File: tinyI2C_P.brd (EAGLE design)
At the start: 80.8 x 80 mm, 224 parts, among them IC1 74ABT125BQ, IC10 74ABT125BQ, IC11 TPS76318, IC12 74ABT125BQ, IC13 TPS76318, IC14 74ABT125BQ, IC15 TPS76318, IC16 74ABT125BQ, IC2 TPS76318, IC3 TPS76318, IC4 74ABT125BQ, IC5 TPS76318, IC6 74ABT125BQ, IC7 TPS76318, IC8 74ABT125BQ, IC9 TPS76318, U1 LPC824M201JHI33, U2 LPC824M201JHI33, U3 LPC824M201JHI33, U4 LPC824M201JHI33, U5 LPC824M201JHI33, U6 LPC824M201JHI33, U7 LPC824M201JHI33, U8 LPC824M201JHI33, X1 TSW-112-02-S-S, X10 TSW-112-02-S-S, X11 TSW-112-02-S-S, X12 TSW-102-02-S-S, X13 TSW-106-02-S-S-RA, X14 TSW-112-02-S-S, X15 TSW-112-02-S-S, X16 TSW-102-02-S-S, X17 TSW-106-02-S-S-RA, X18 TSW-112-02-S-S, X19 TSW-112-02-S-S, X2 TSW-106-02-S-S-RA, X20 TSW-102-02-S-S, X21 TSW-106-02-S-S-RA, X22 TSW-112-02-S-S, X23 TSW-112-02-S-S, X24 TSW-102-02-S-S, X25 TSW-106-02-S-S-RA, X26 TSW-112-02-S-S, X27 TSW-112-02-S-S, X28 TSW-102-02-S-S, X29 TSW-106-02-S-S-RA, X3 TSW-112-02-S-S, X30 TSW-112-02-S-S, X31 TSW-112-02-S-S, X32 TSW-102-02-S-S, X4 TSW-102-02-S-S, X5 TSW-106-02-S-S-RA, X6 TSW-112-02-S-S, X7 TSW-112-02-S-S, X8 TSW-102-02-S-S, X9 TSW-106-02-S-S-RA

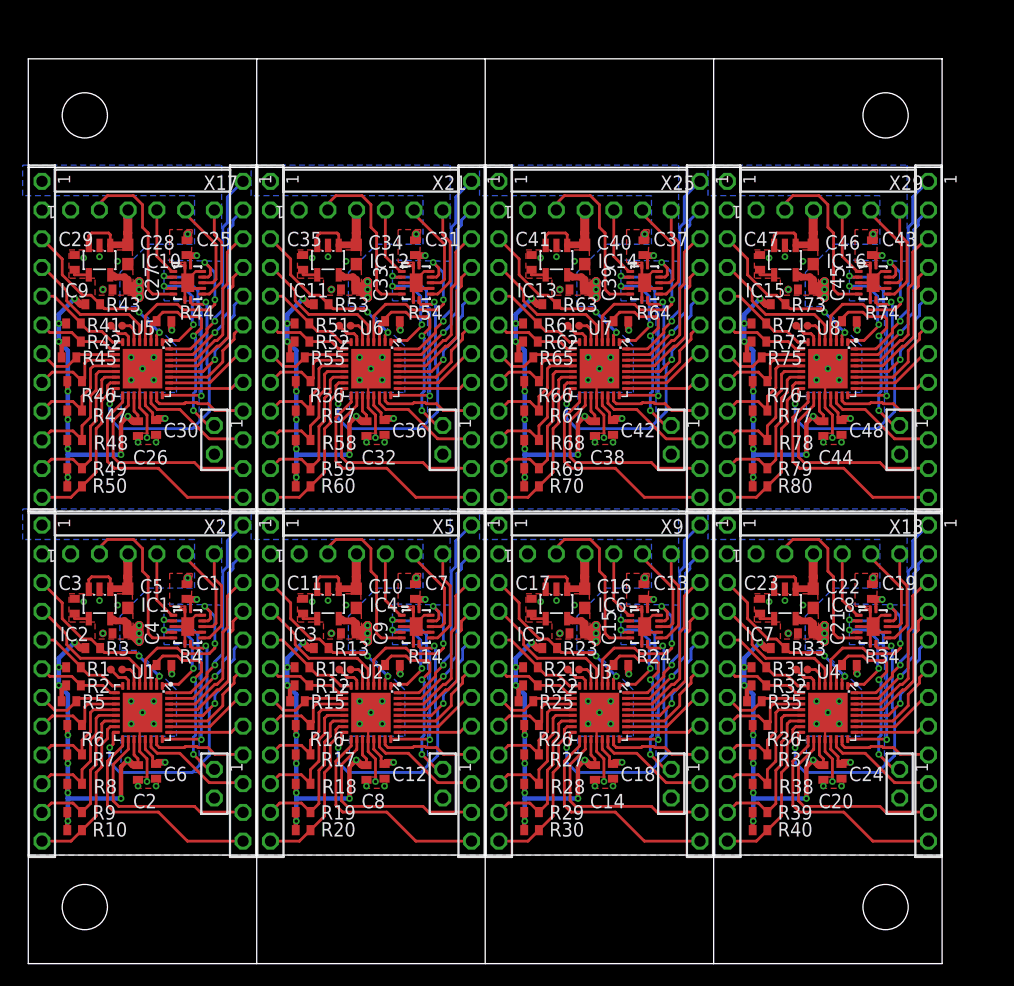
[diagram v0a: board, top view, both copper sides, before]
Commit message: [ GERBER ] update
panelized
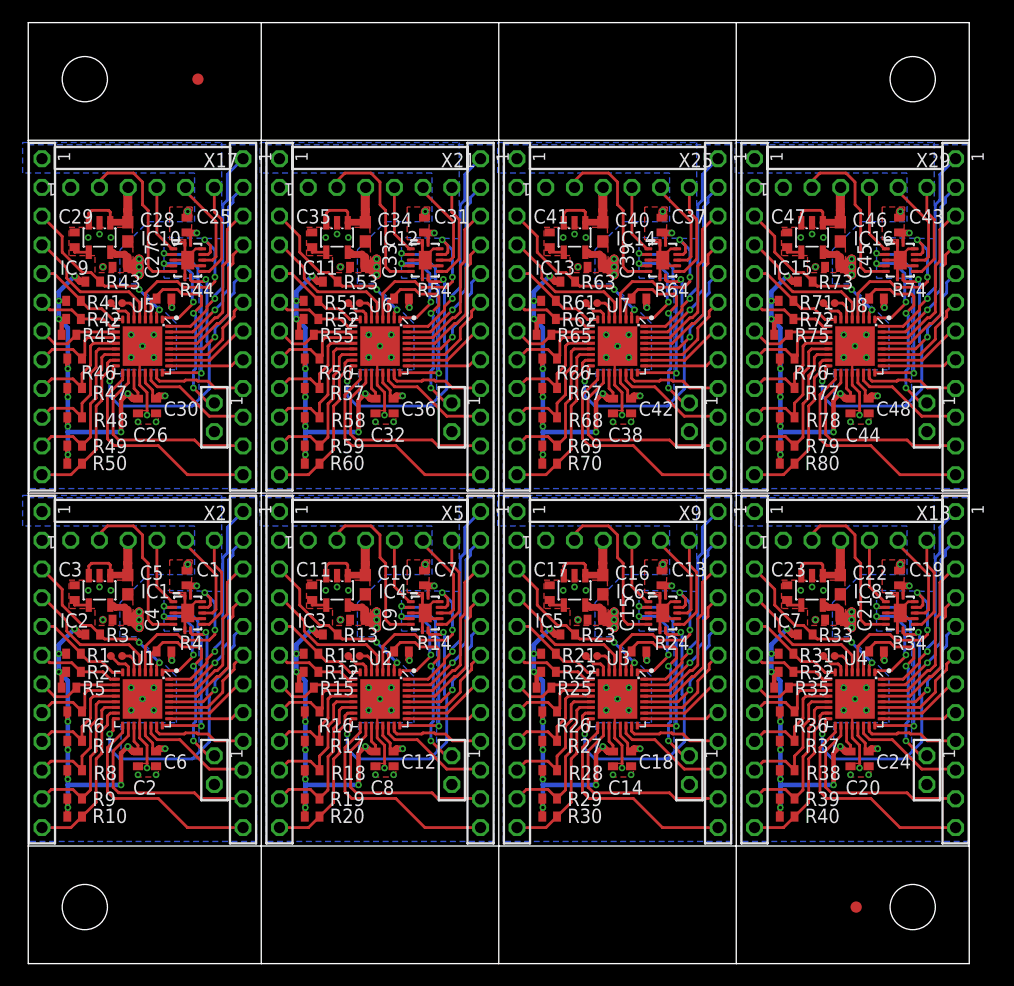
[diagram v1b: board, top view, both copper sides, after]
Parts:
- added TP41, TP42: TPTP07R, testpad:TP07R
- TP4, TP5: value TPTP07R -> TPTP10R; device testpad:TP07R -> testpad:TP10R
- moved TP21 72.0 mm to (70.3, 27.2)
- moved TP22 68.2 mm to (69.6, 30.4)
- moved TP5 51.2 mm to (73.2, 5.00)
- moved TP4 46.2 mm to (15.0, 78.2)
- moved TP26 22.6 mm to (7.30, 58.4)
- moved TP27 22.1 mm to (6.60, 61.6)
- moved TP11 22.0 mm to (28.3, 27.2)
- moved TP31 21.8 mm to (28.3, 58.4)
- moved TP32 21.3 mm to (27.6, 61.6)
- moved TP12 21.3 mm to (27.6, 30.4)
- moved TP16 21.3 mm to (49.3, 27.2)
- moved TP36 21.0 mm to (49.3, 58.4)
- moved TP37 20.5 mm to (48.6, 61.6)
- moved TP17 20.5 mm to (48.6, 30.4)
- moved TP38 10.6 mm to (71.8, 66.6)
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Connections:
- net 1.8V1: now also TP7.TP; no longer TP5.TP
- net 1.8V2: now also TP14.TP; no longer TP12.TP
- net 1.8V3: now also TP19.TP; no longer TP17.TP
- net 1.8V4: now also TP24.TP; no longer TP22.TP
- net 1.8V5: now also TP29.TP; no longer TP27.TP
- net 1.8V6: now also TP34.TP; no longer TP32.TP
- net 1.8V7: now also TP39.TP; no longer TP37.TP
- net 5V1: now also TP6.TP; no longer TP4.TP
- net 5V2: now also TP13.TP; no longer TP11.TP
- net 5V3: now also TP18.TP; no longer TP16.TP
- net 5V4: now also TP23.TP; no longer TP21.TP
- net 5V5: now also TP28.TP; no longer TP26.TP
- net 5V6: now also TP33.TP; no longer TP31.TP
- net 5V7: now also TP38.TP; no longer TP36.TP
- net GND1: now also TP12.TP; no longer TP10.TP
- net GND2: now also TP17.TP; no longer TP15.TP
- net GND3: now also TP22.TP; no longer TP20.TP
- net GND4: now also TP27.TP; no longer TP25.TP
- net GND5: now also TP32.TP; no longer TP30.TP
- net GND6: now also TP37.TP; no longer TP35.TP
- net GND7: now also TP42.TP; no longer TP40.TP
- net SWCLK1: now also TP10.TP; no longer TP6.TP
- net SWCLK2: now also TP15.TP; no longer TP13.TP
- net SWCLK3: now also TP20.TP; no longer TP18.TP
- net SWCLK4: now also TP25.TP; no longer TP23.TP
- net SWCLK5: now also TP30.TP; no longer TP28.TP
- net SWCLK6: now also TP35.TP; no longer TP33.TP
- net SWCLK7: now also TP40.TP; no longer TP38.TP
- net SWDIO1: now also TP11.TP; no longer TP7.TP
- net SWDIO2: now also TP16.TP; no longer TP14.TP
- net SWDIO3: now also TP21.TP; no longer TP19.TP
- net SWDIO4: now also TP26.TP; no longer TP24.TP
- net SWDIO5: now also TP31.TP; no longer TP29.TP
- net SWDIO6: now also TP36.TP; no longer TP34.TP
- net SWDIO7: now also TP41.TP; no longer TP39.TP
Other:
- board size 80.8 x 80 mm -> 83.2 x 83.2 mm
